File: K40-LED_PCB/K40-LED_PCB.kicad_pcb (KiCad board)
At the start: 2 copper layers, 27.8 x 27.8 mm, 14 parts, among them p1 12V_Pad

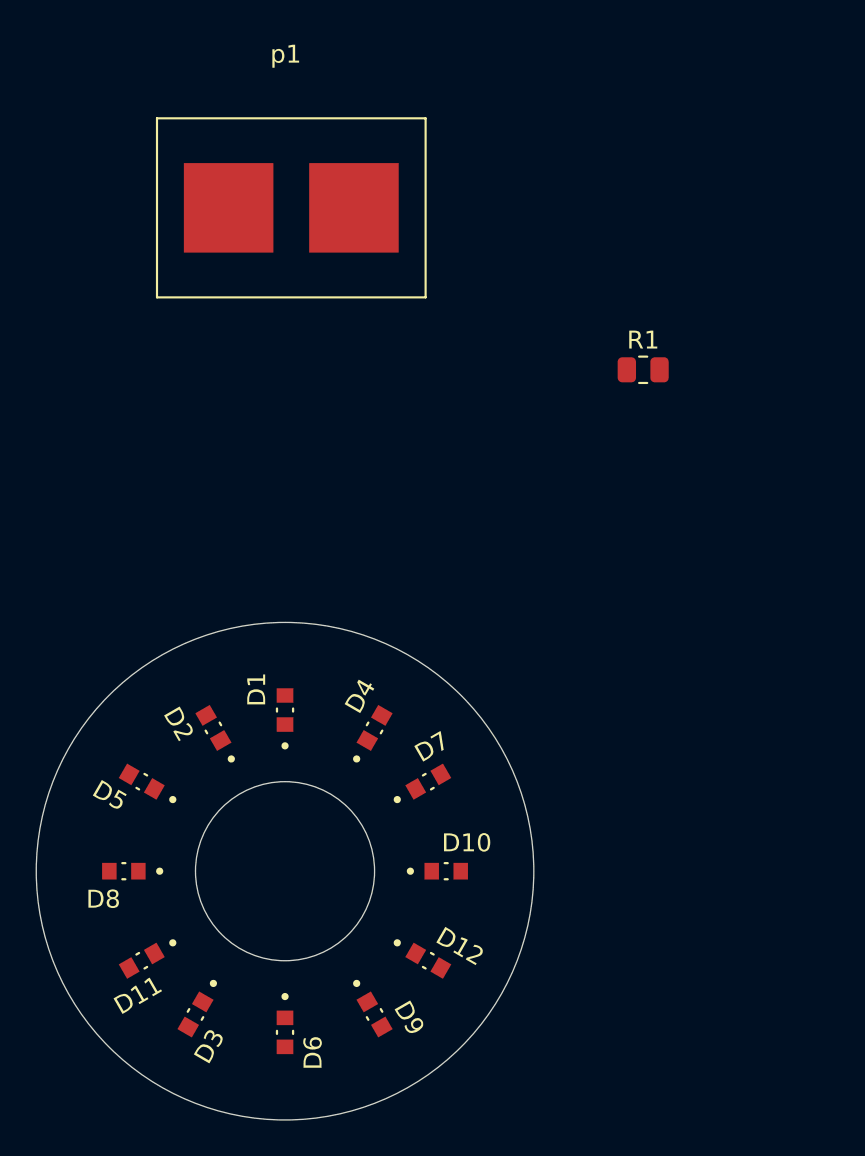
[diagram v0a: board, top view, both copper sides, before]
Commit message: PCb_Complete
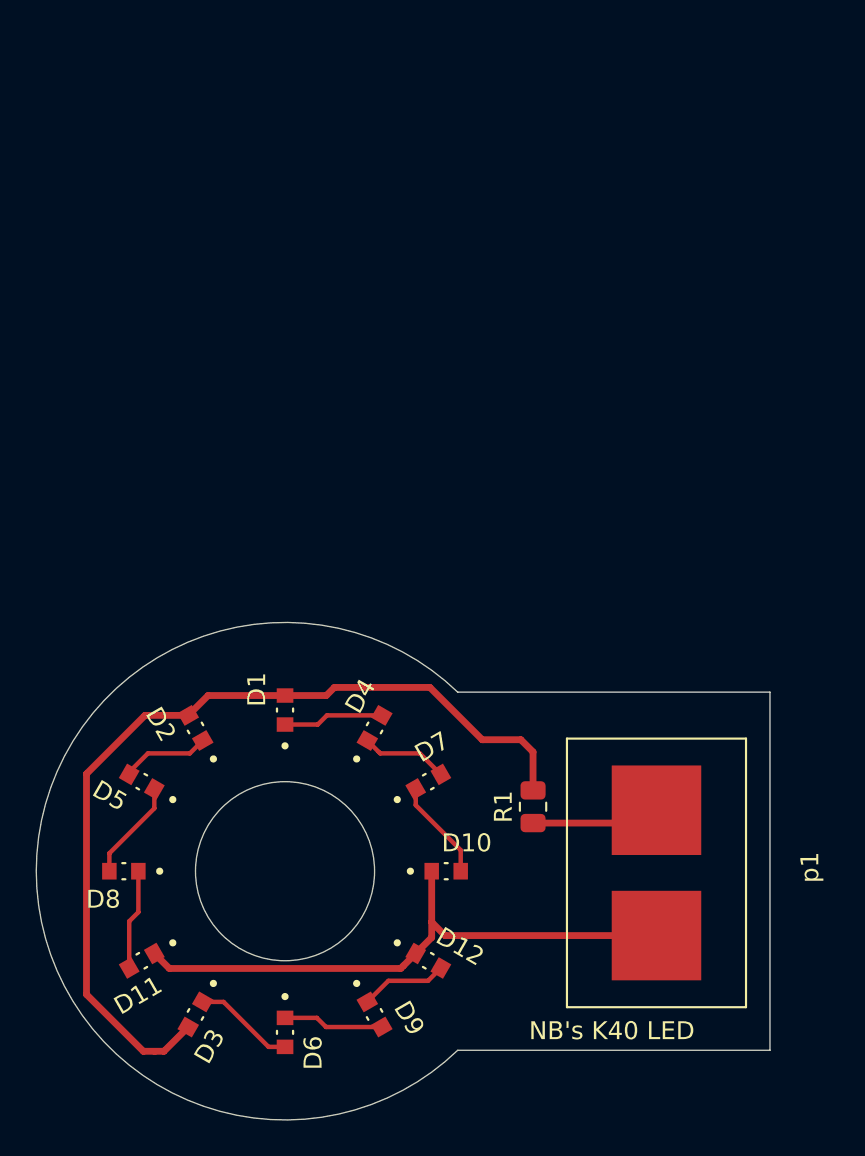
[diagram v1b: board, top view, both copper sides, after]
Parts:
- moved p1 47.8 mm to (102.7, 65.6), turned to 270 degrees
- moved R1 25.2 mm to (90.8, 69.4), turned to 90 degrees
- moved D2 1.00 mm to (72.0, 65.0)
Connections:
- D10 pad C: GND -> Net-(D10-PadC)
- D11 pad C: GND -> Net-(D10-PadC)
- D12 pad C: GND -> Net-(D10-PadC)
- p1 pad 2: Net-(p1-Pad2) -> Net-(D10-PadC)
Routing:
- net Net-(D1-PadA): track 0.00 -> 50.5 mm
- net Net-(D10-PadC): track 0.00 -> 33.1 mm
- net Net-(R1-Pad1): track 0.00 -> 7.19 mm
- net Net-(D5-PadC): track 0.00 -> 5.64 mm
- net Net-(D3-PadC): track 0.00 -> 5.64 mm
- net Net-(D10-PadA): track 0.00 -> 5.64 mm
- net Net-(D11-PadA): track 0.00 -> 5.62 mm
- net Net-(D6-PadC): track 0.00 -> 5.62 mm
- net Net-(D1-PadC): track 0.00 -> 5.62 mm
- net Net-(D2-PadC): track 0.00 -> 4.97 mm
- net Net-(D12-PadA): track 0.00 -> 4.89 mm
- net Net-(D4-PadC): track 0.00 -> 4.89 mm
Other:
- board size 27.8 x 27.8 mm -> 41 x 27.8 mm
- board text added: "NB's K40 LED"
